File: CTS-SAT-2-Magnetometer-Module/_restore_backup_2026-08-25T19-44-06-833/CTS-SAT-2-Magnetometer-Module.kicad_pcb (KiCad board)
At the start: 6 copper layers, 39.3 x 27.5 mm, 32 parts, among them J1 Conn_01x04_Pin, J2 SWD, SW1 SW_Push, U1 MMC5983MA, U2 LIS2MDL, U3 STM32F072C8Tx, U5 MIC5365-3.0YC5

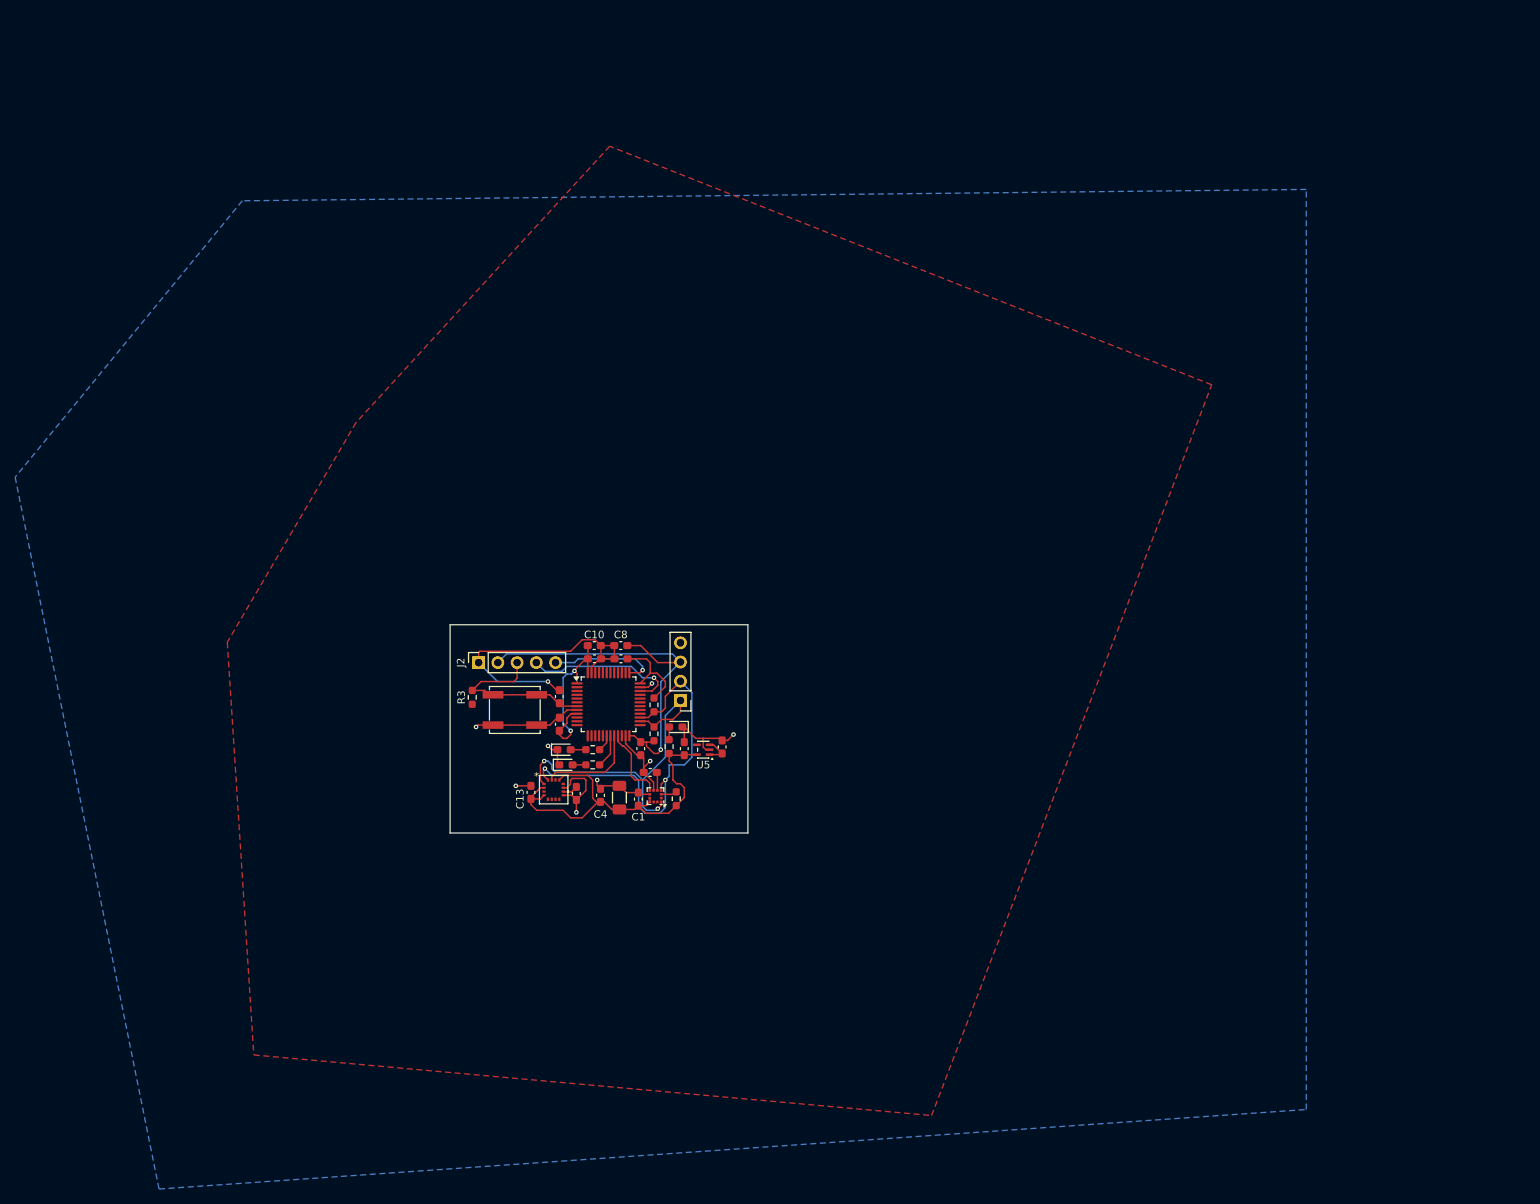
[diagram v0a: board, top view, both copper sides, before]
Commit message: Complete Routing
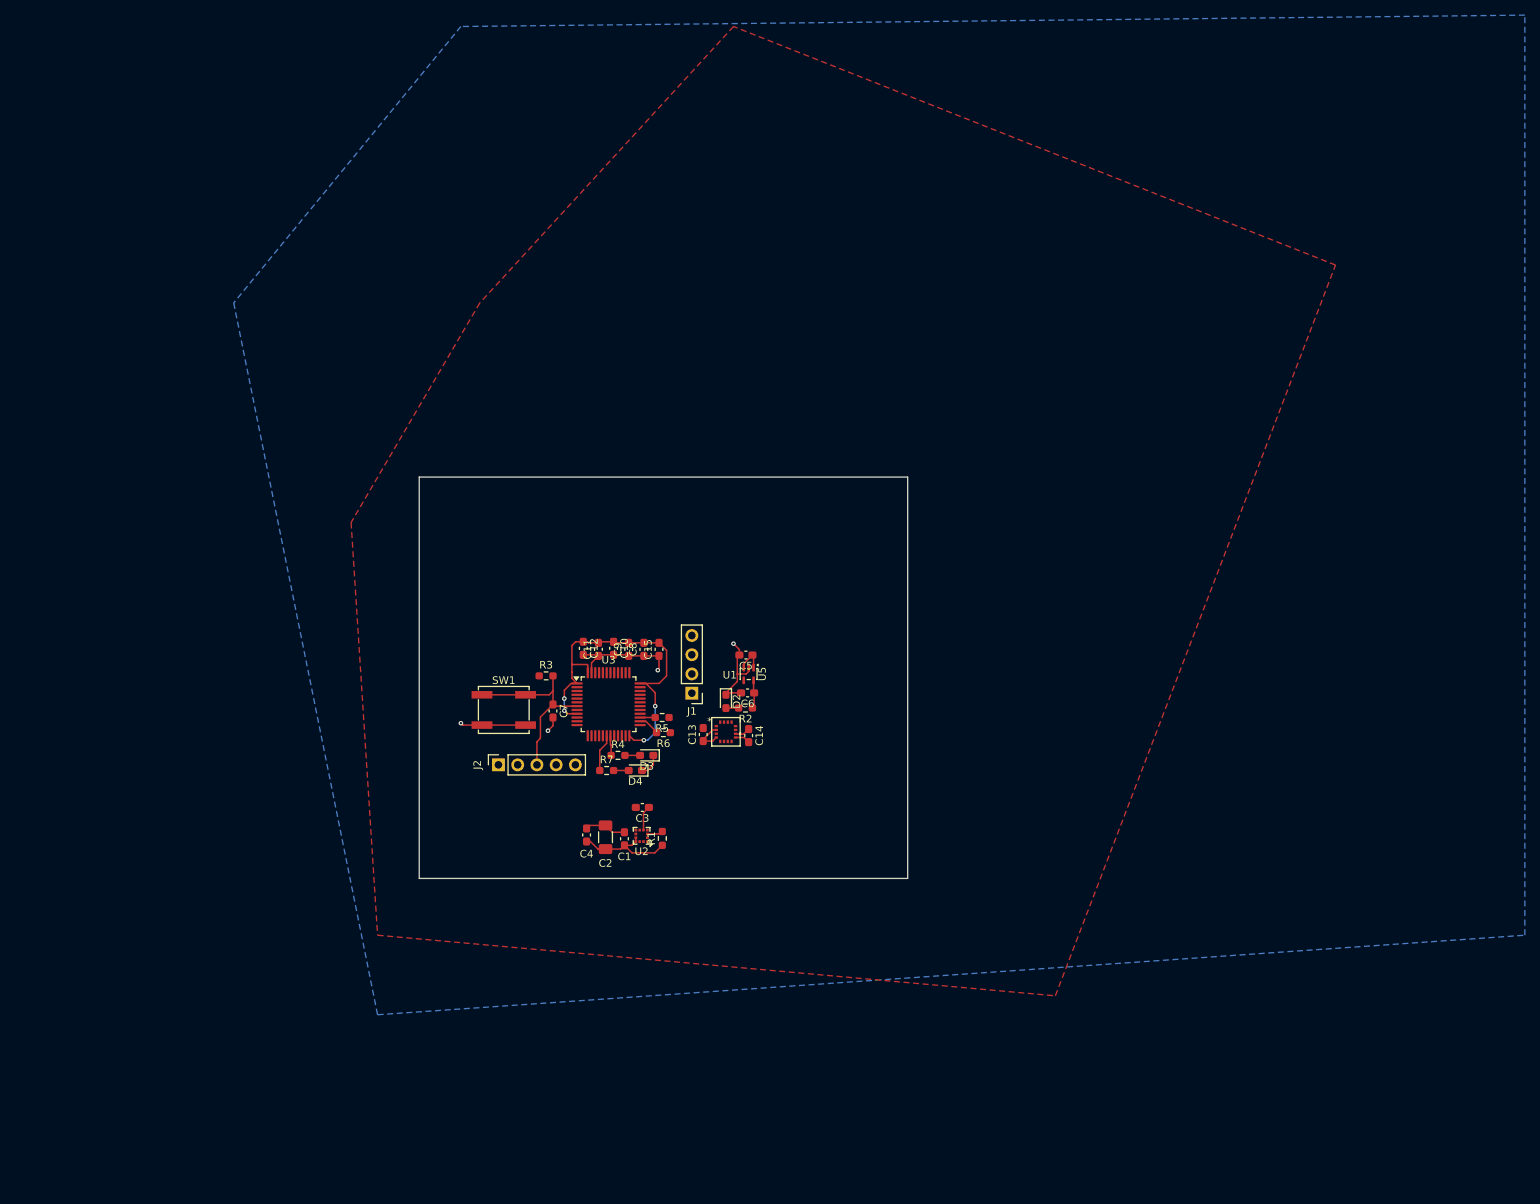
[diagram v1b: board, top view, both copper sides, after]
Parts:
- moved C14 24.0 mm to (140.5, 122.1)
- moved U1 24.0 mm to (137.5, 121.6)
- moved C13 24.0 mm to (134.5, 122.0)
- moved J2 13.8 mm to (107.5, 126.0)
- moved C15 13.3 mm to (128.7, 110.8)
- moved C5 12.5 mm to (140.1, 111.5), turned to 180 degrees
- moved U5 11.7 mm to (140.5, 114.0), turned to -90 degrees
- moved R2 11.3 mm to (140.1, 118.5), turned to 180 degrees
- moved C6 11.1 mm to (140.4, 116.5), turned to 180 degrees
- moved D3 10.7 mm to (127.0, 124.8), turned to 180 degrees
- moved C12 10.5 mm to (118.7, 110.6), turned to -90 degrees
- moved R3 10.2 mm to (113.8, 114.2), turned to 0 degrees
- moved D4 9.81 mm to (125.5, 126.8), turned to 180 degrees
- moved D2 7.44 mm to (137.5, 117.6), turned to -90 degrees
- moved C2 5.55 mm to (121.6, 135.6)
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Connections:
- J1 pad 3: +3V3 -> 3V3
- J2 pad 2: +3V3 -> 3V3
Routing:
- net GND: track 103.9 -> 48.0 mm, vias 9 -> 4
- net SDA: track 52.3 -> 2.00 mm, vias 2 -> 0
- net SCL: track 45.2 -> 2.85 mm, vias 2 -> 0
- net +3V3: track 87.8 -> 46.6 mm, vias 3 -> 4
- net +3V0: track 50.4 -> 21.8 mm
- net SWDIO: track 20.8 -> 0.00 mm, vias 1 -> 0
- net SWCLK: track 14.5 -> 0.00 mm, vias 1 -> 0
- net INT: track 13.1 -> 0.00 mm
- net DRDY: track 9.94 -> 0.00 mm
- net Net-(U3-PB0): track 2.22 -> 4.97 mm
- net NRST: track 23.4 -> 25.5 mm
- net Net-(U3-PB1): track 4.43 -> 2.62 mm
- net Net-(U2-C1): track 2.41 -> 3.28 mm
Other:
- board size 39.3 x 27.5 mm -> 64.5 x 53 mm
